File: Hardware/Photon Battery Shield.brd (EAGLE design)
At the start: 20.3 x 40.6 mm, 14 parts, among them J1 POWER_JACKSMD, U1 MCP73831, U2 MAX1704X

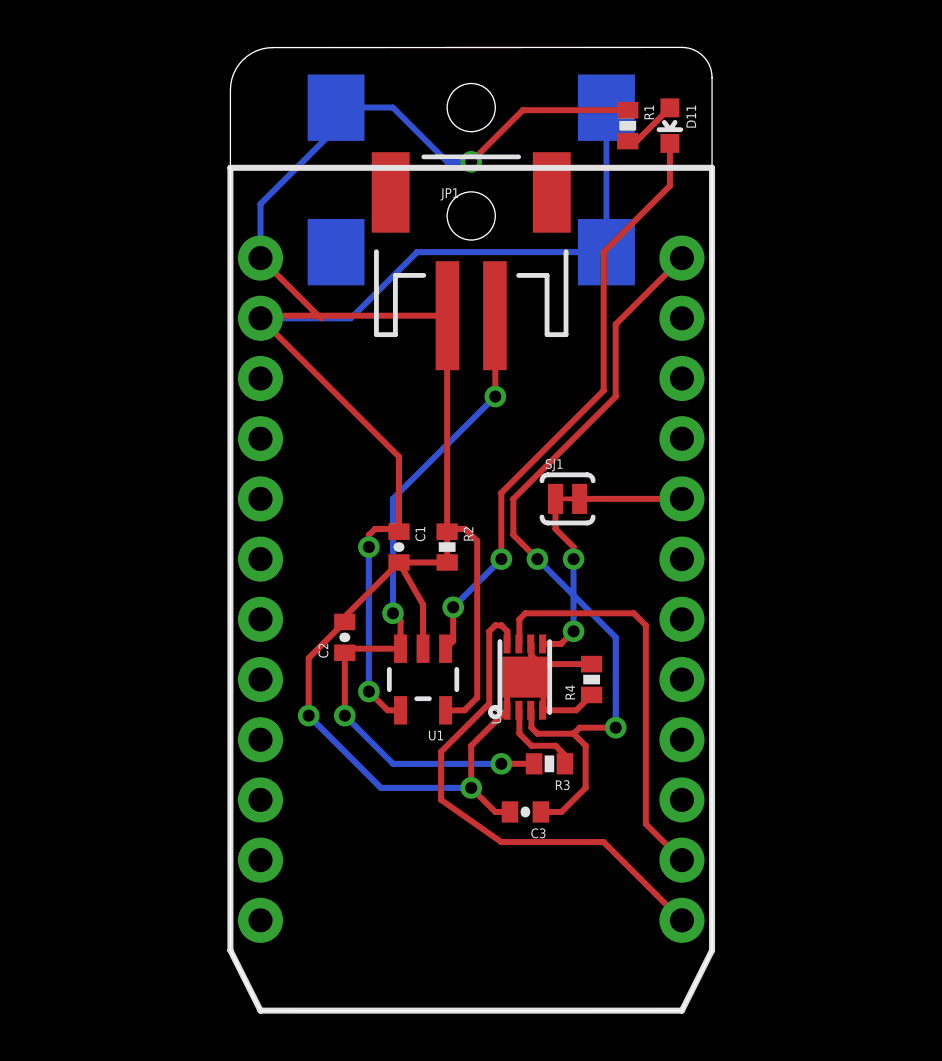
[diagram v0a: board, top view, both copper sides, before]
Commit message: Re-layed out, needs traces done
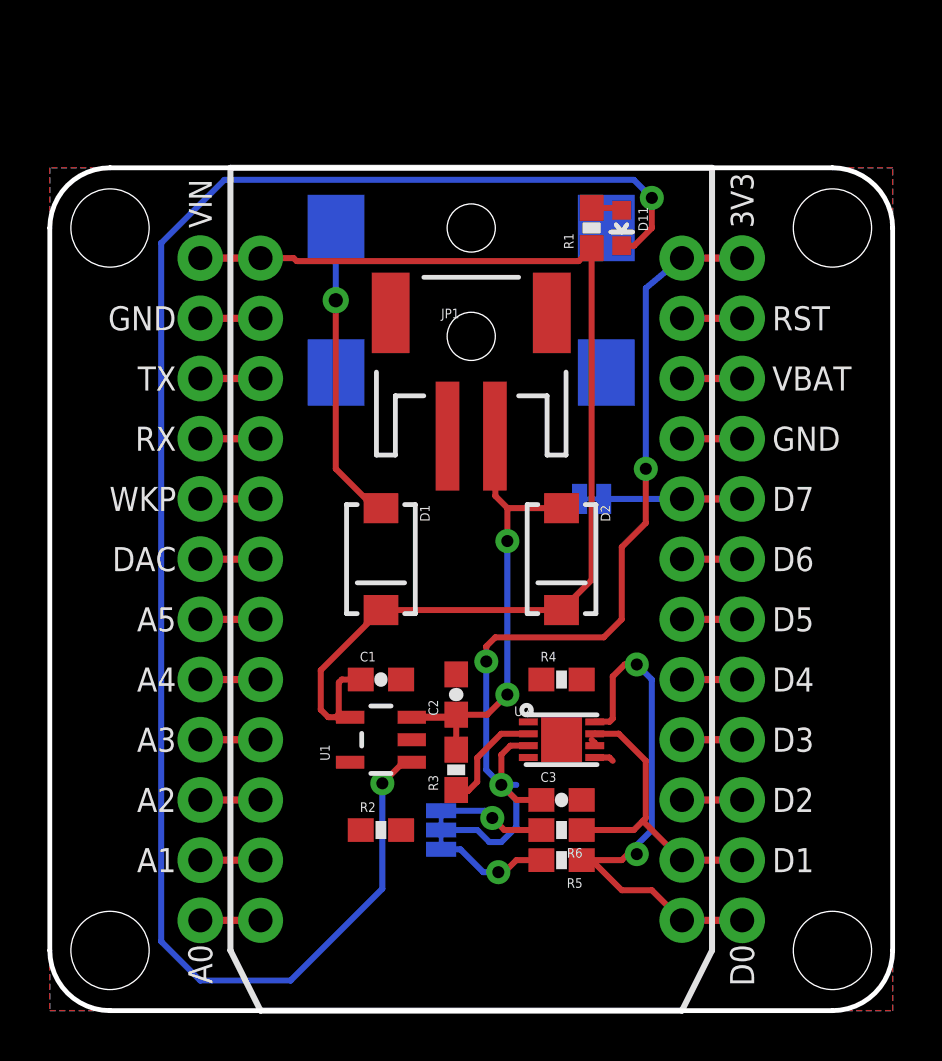
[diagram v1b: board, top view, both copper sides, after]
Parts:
- added D1, D2: MBRA140, SparkFun-DiscreteSemi:SMA-DIODE
- added R5, R6: 10K, SparkFun-Resistors:0603-RES
- added SJ2: (no value), SparkFun-Passives:PAD-JUMPER-3-3OF3_NC_BY_TRACE_YES_SILK_FULL_BOX
- C1, C2: value 4.7uf -> 4.7uF; device SparkFun-Passives:0402-CAP -> SparkFun-Passives:0603-CAP
- C3: device SparkFun-Passives:0402-CAP -> SparkFun-Passives:0603-CAP
- JP3: value SPARK_PHOTON -> SPARK_PHOTONTEMPLATE; device template_temp:SPARK_PHOTON -> template_temp:SPARK_PHOTON_TEMPLATE
- R1, R2, R3, R4: device SparkFun-Passives:0402-RES -> SparkFun-Passives:0603-RES
- moved R2 12.3 mm to (6.35, 7.62), turned to 0 degrees
- moved C1 5.64 mm to (6.35, 14.0), turned to 0 degrees
- moved C2 5.28 mm to (9.53, 13.3)
- moved JP1 5.08 mm to (10.2, 27.9)
- moved J1 5.08 mm to (10.2, 33.0)
- moved D11 4.77 mm to (16.5, 33.0)
- moved R1 4.58 mm to (15.2, 33.0), turned to 90 degrees
- moved R3 3.95 mm to (9.53, 10.2), turned to 90 degrees
- moved U1 3.10 mm to (6.35, 11.4), turned to 90 degrees
- moved U2 3.06 mm to (14.0, 11.4), turned to 0 degrees
- moved C3 1.61 mm to (14.0, 8.89), turned to 0 degrees
- moved R4 1.27 mm to (14.0, 14.0), turned to 0 degrees
- moved SJ1 1.02 mm to (15.2, 21.6), flipped to the bottom, turned to 180 degrees
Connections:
- new net N$7: R5.2, SJ2.3
- new net N$8: D1.A, J1.VIN0
- new net N$9: R6.2, SJ2.1
- net 3.3V: now also JP3.3V3, SJ2.2
- net D7: now also JP3.D7
- net GND: now also JP3.GND@0
- net SCL: now also JP3.D1, R6.1
- net SDA: now also JP3.D0, R5.1
- net VBAT: now also D2.A
- net VIN: now also D1.C, D2.C, JP3.VIN; no longer J1.VIN0
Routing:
- net GND: track 74.8 -> 0.00 mm, vias 2 -> 0
- net N$2: track 25.2 -> 72.1 mm
- net N$8: track 0.00 -> 12.8 mm, vias 0 -> 1
- net VBAT: track 29.9 -> 19.3 mm, vias 4 -> 2
- net N$3: track 9.69 -> 0.00 mm
- net SCL: track 17.2 -> 10.3 mm
- net N$4: track 7.43 -> 0.82 mm, vias 2 -> 0
- net 3.3V: track 33.9 -> 39.5 mm, vias 2 -> 3
- net N$7: track 0.00 -> 4.84 mm, vias 0 -> 1
- net N$9: track 0.00 -> 4.57 mm, vias 0 -> 1
- net N$6: track 3.19 -> 0.30 mm
- net SDA: track 21.6 -> 20.1 mm, vias 0 -> 2
- net N$1: track 2.36 -> 1.31 mm
- net D7: track 4.32 -> 3.30 mm
- net N$5: track 3.66 -> 4.65 mm
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- added copper zone on layer 1, net GND
- added copper zone on layer 16, net GND
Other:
- board size 20.3 x 40.6 mm -> 35.6 x 35.6 mm
